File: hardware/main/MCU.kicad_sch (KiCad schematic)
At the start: 17 parts, among them U1 NUCLEO64-F411RE

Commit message: added status LED's to schema, fixed gate drive error, added BOM
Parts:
- R21, R22, R30, R31, R32, R33, R34, R35, R36, R37, R38, R39, R40, R41, R42: footprint (none) -> Resistor_SMD:R_0402_1005Metric
- RV1: footprint (none) -> Potentiometer_THT:Potentiometer_Alps_RK09K_Single_Vertical
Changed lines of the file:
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@@
 			)
 		)
-		(property "Footprint" ""
+		(property "Footprint" "Resistor_SMD:R_0402_1005Metric"
 			(at 232.41 55.118 90)
 			(hide yes)
@@
 			)
 		)
-		(property "Footprint" ""
+		(property "Footprint" "Resistor_SMD:R_0402_1005Metric"
 			(at 234.95 117.348 90)
 			(hide yes)
@@
 			)
 		)
-		(property "Footprint" ""
+		(property "Footprint" "Potentiometer_THT:Potentiometer_Alps_RK09K_Single_Vertical"
 			(at 254 144.78 0)
 			(hide yes)
@@
 			)
 		)
-		(property "Footprint" ""
+		(property "Footprint" "Resistor_SMD:R_0402_1005Metric"
 			(at 234.95 112.268 90)
 			(hide yes)
@@
 			)
 		)
-		(property "Footprint" ""
+		(property "Footprint" "Resistor_SMD:R_0402_1005Metric"
 			(at 234.95 102.108 90)
 			(hide yes)
@@
 			)
 		)
-		(property "Footprint" ""
+		(property "Footprint" "Resistor_SMD:R_0402_1005Metric"
 			(at 234.95 84.328 90)
 			(hide yes)
@@
 			)
 		)
-		(property "Footprint" ""
+		(property "Footprint" "Resistor_SMD:R_0402_1005Metric"
 			(at 232.41 39.878 90)
 			(hide yes)
@@
 			)
 		)
-		(property "Footprint" ""
+		(property "Footprint" "Resistor_SMD:R_0402_1005Metric"
 			(at 232.41 50.038 90)
 			(hide yes)
@@
 			)
 		)
-		(property "Footprint" ""
+		(property "Footprint" "Resistor_SMD:R_0402_1005Metric"
 			(at 232.41 29.718 90)
 			(hide yes)
@@
 			)
 		)
-		(property "Footprint" ""
+		(property "Footprint" "Resistor_SMD:R_0402_1005Metric"
 			(at 223.52 146.558 90)
 			(hide yes)
@@
 			)
 		)
-		(property "Footprint" ""
+		(property "Footprint" "Resistor_SMD:R_0402_1005Metric"
 			(at 234.95 89.408 90)
 			(hide yes)
@@
 			)
 		)
-		(property "Footprint" ""
+		(property "Footprint" "Resistor_SMD:R_0402_1005Metric"
 			(at 232.41 44.958 90)
 			(hide yes)
@@
 			)
 		)
-		(property "Footprint" ""
+		(property "Footprint" "Resistor_SMD:R_0402_1005Metric"
 			(at 232.41 67.818 90)
 			(hide yes)
@@
 			)
 		)
-		(property "Footprint" ""
+		(property "Footprint" "Resistor_SMD:R_0402_1005Metric"
 			(at 234.95 107.188 90)
 			(hide yes)
@@
 			)
 		)
-		(property "Footprint" ""
+		(property "Footprint" "Resistor_SMD:R_0402_1005Metric"
 			(at 232.41 34.798 90)
 			(hide yes)
@@
 			)
 		)
-		(property "Footprint" ""
+		(property "Footprint" "Resistor_SMD:R_0402_1005Metric"
 			(at 234.95 79.248 90)
 			(hide yes)

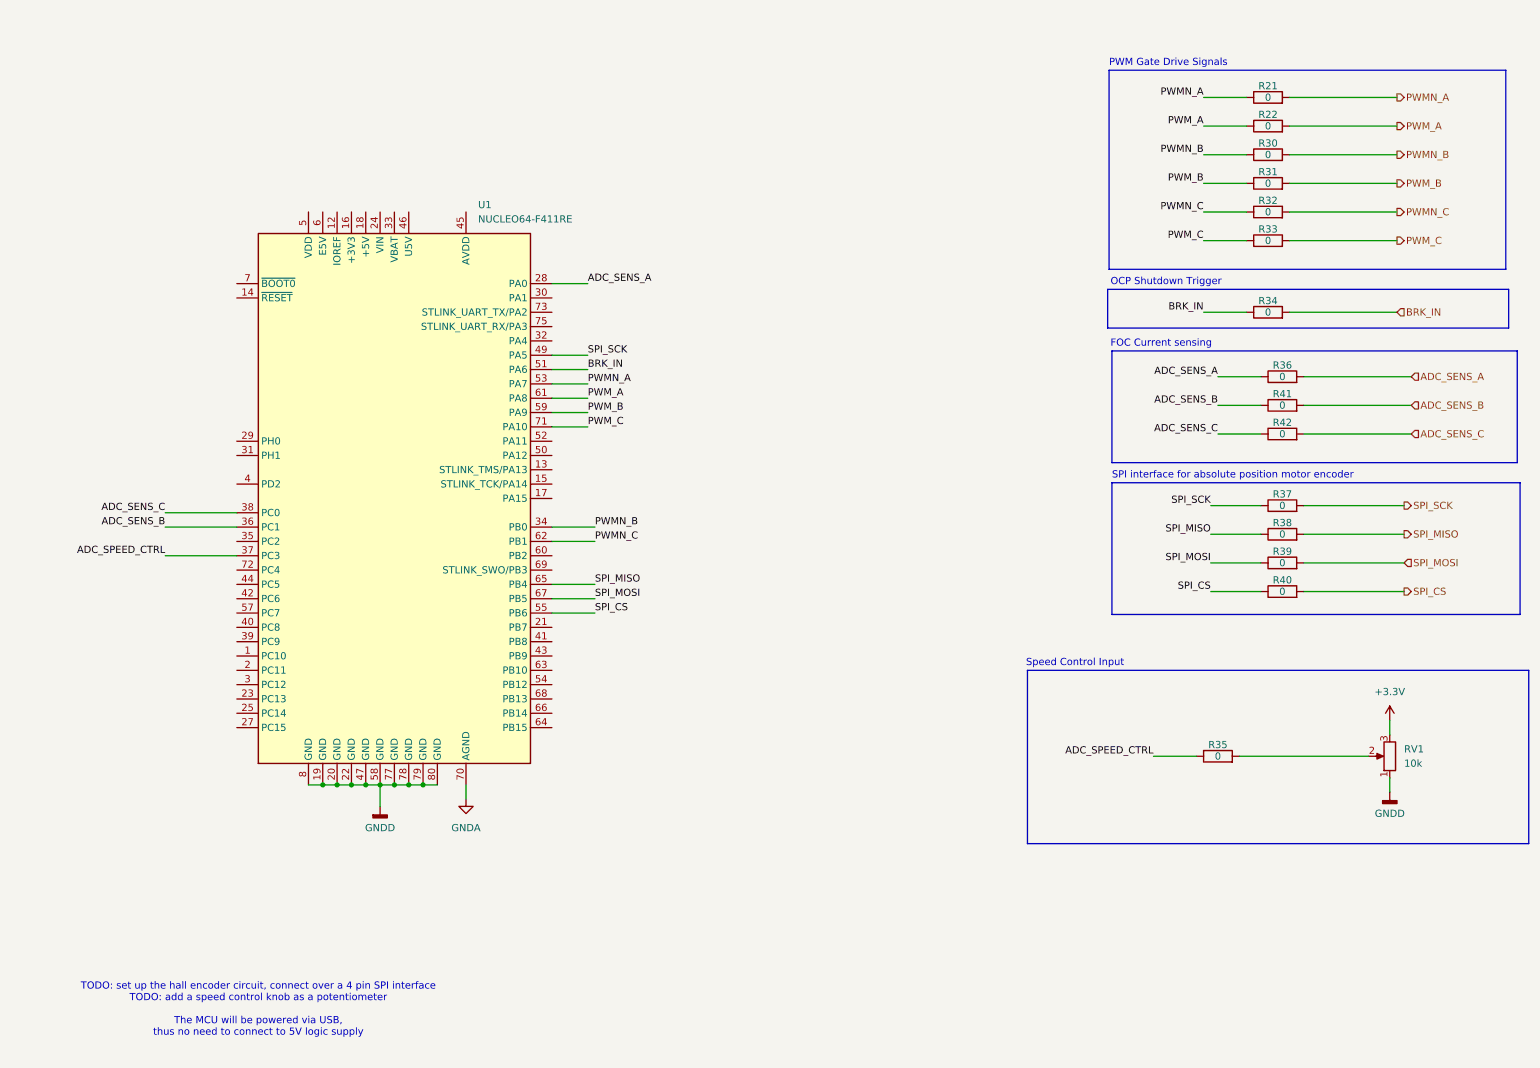
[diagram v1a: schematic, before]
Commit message: hardware layout started
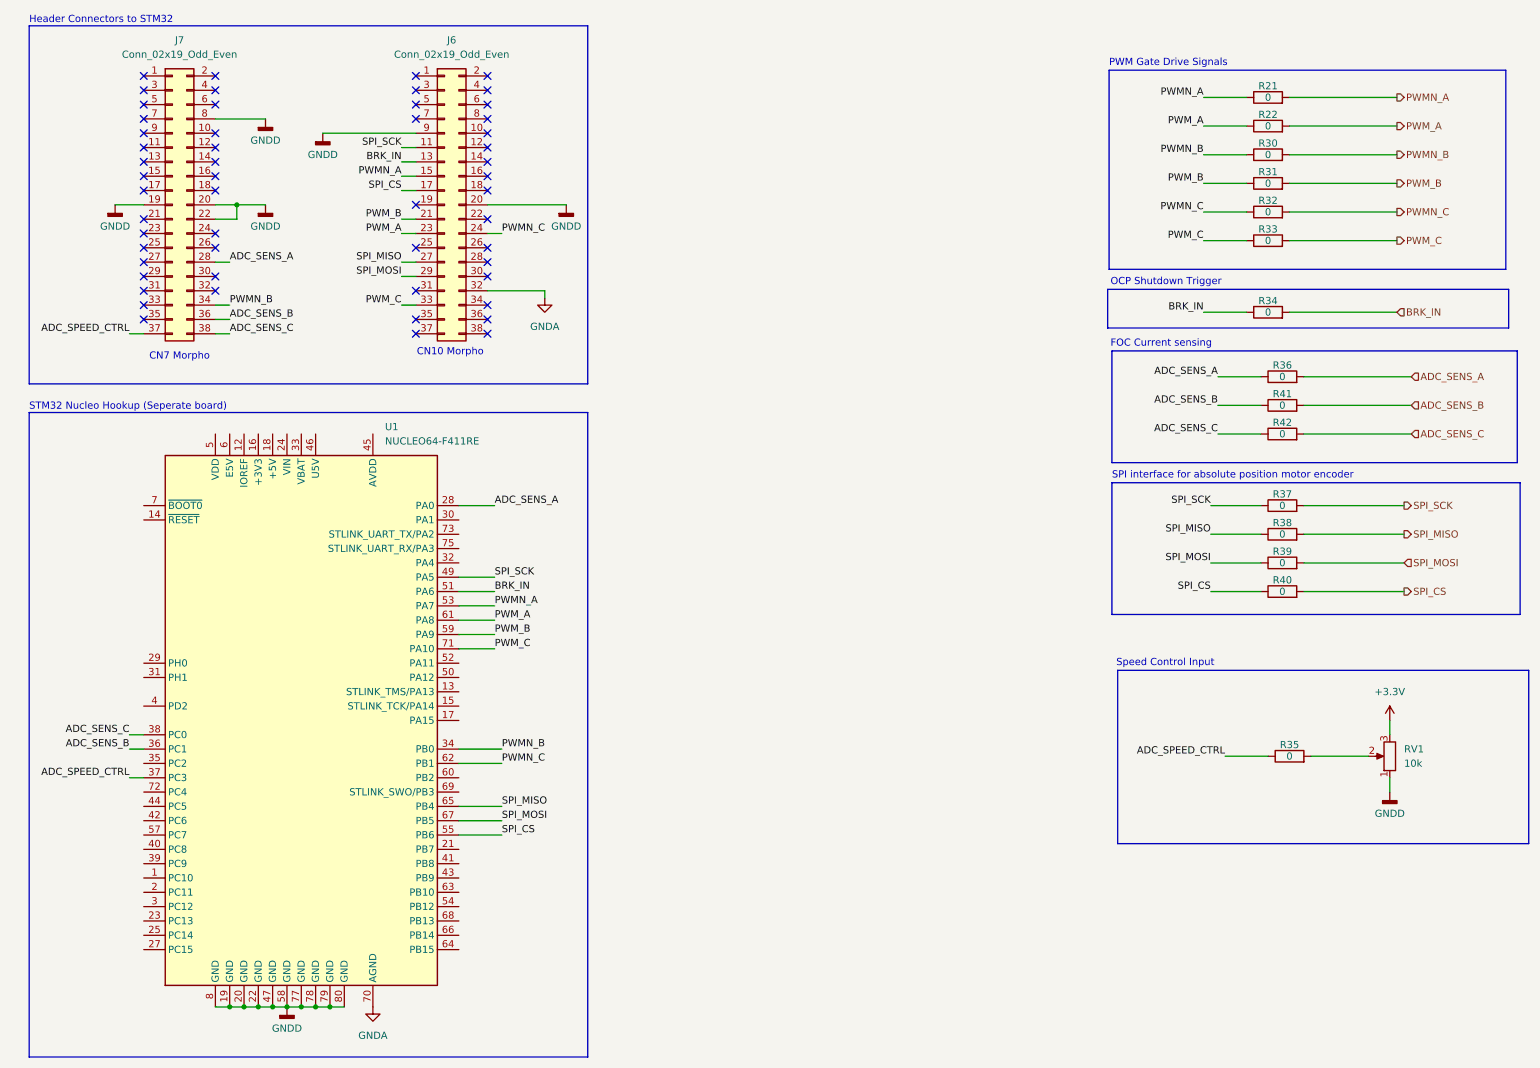
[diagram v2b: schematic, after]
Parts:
- added J6, J7: Conn_02x19_Odd_Even, Connector_PinSocket_2.54mm:PinSocket_2x19_P2.54mm_Vertical, symbol Connector_Generic:Conn_02x19_Odd_Even
- U1: now left out of the parts list
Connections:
- net ADC_SENS_A: now also J7.28 (Pin_28)
- net ADC_SENS_B: now also J7.36 (Pin_36)
- net ADC_SENS_C: now also J7.38 (Pin_38)
- net ADC_SPEED_CTRL: now also J7.37 (Pin_37)
- net BRK_IN: now also J6.13 (Pin_13)
- net GNDA: now also J6.32 (Pin_32)
- net GNDD: now also J6.20 (Pin_20), J6.9 (Pin_9), J7.19 (Pin_19), J7.20 (Pin_20), J7.22 (Pin_22), J7.8 (Pin_8)
- net PWMN_A: now also J6.15 (Pin_15)
- net PWMN_B: now also J7.34 (Pin_34)
- net PWMN_C: now also J6.24 (Pin_24)
- net PWM_A: now also J6.23 (Pin_23)
- net PWM_B: now also J6.21 (Pin_21)
- net PWM_C: now also J6.33 (Pin_33)
- net SPI_CS: now also J6.17 (Pin_17)
- net SPI_MISO: now also J6.27 (Pin_27)
- net SPI_MOSI: now also J6.29 (Pin_29)
- net SPI_SCK: now also J6.11 (Pin_11)
- no-connect marks 0 -> 54
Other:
- note added: "CN10 Morpho"
- note added: "CN7 Morpho"
- note added: "Header Connectors to STM32"
- note added: "STM32 Nucleo Hookup (Seperate board)"
- note removed: "TODO: set up the hall encoder circuit, connect over a 4 pin SPI interface TODO: add a speed control knob as a potentiometer The MCU will be powered via USB, thus no need to connect to 5V logic supply"
- moved on the sheet: R35, U1
